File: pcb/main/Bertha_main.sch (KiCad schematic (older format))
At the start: 78 parts, among them J1 RJ12, J12 AudioJack3_SwitchTR, J2 Conn_Coaxial_Power, J3 Conn_02x03_Odd_Even, J4 RJ12, J5 AudioJack3_SwitchTR, J6 SJ, J7 Conn_01x01, J8 Conn_01x01, Q1 ZXMS6004, Q2 ZXMS6004, Q3 MJH6284, Q5 ZXMS6004, Q6 ZXMS6004, Q7 ZXMS6004, U1 DS18B20, U2 ATMEGA32U4-AU, X1 MINI-USB-SCHIELD-32005-201, Y1 Crystal

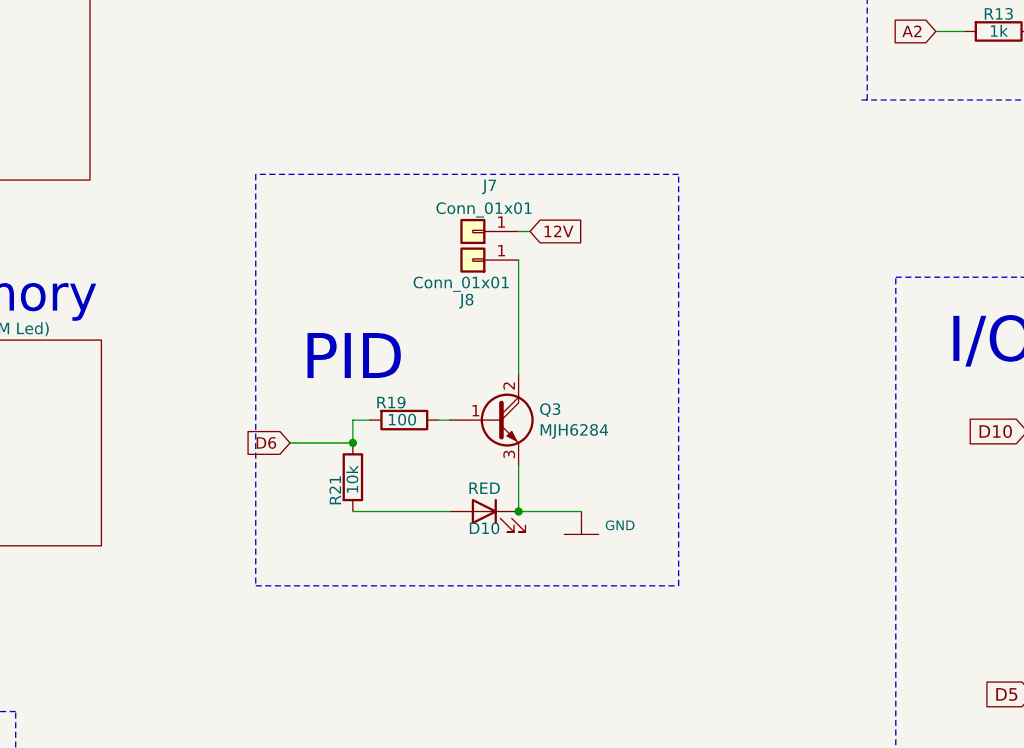
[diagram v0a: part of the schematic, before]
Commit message: Changed MJH6284 darlington transistor for two PB80N03S4L03 MOSFETs
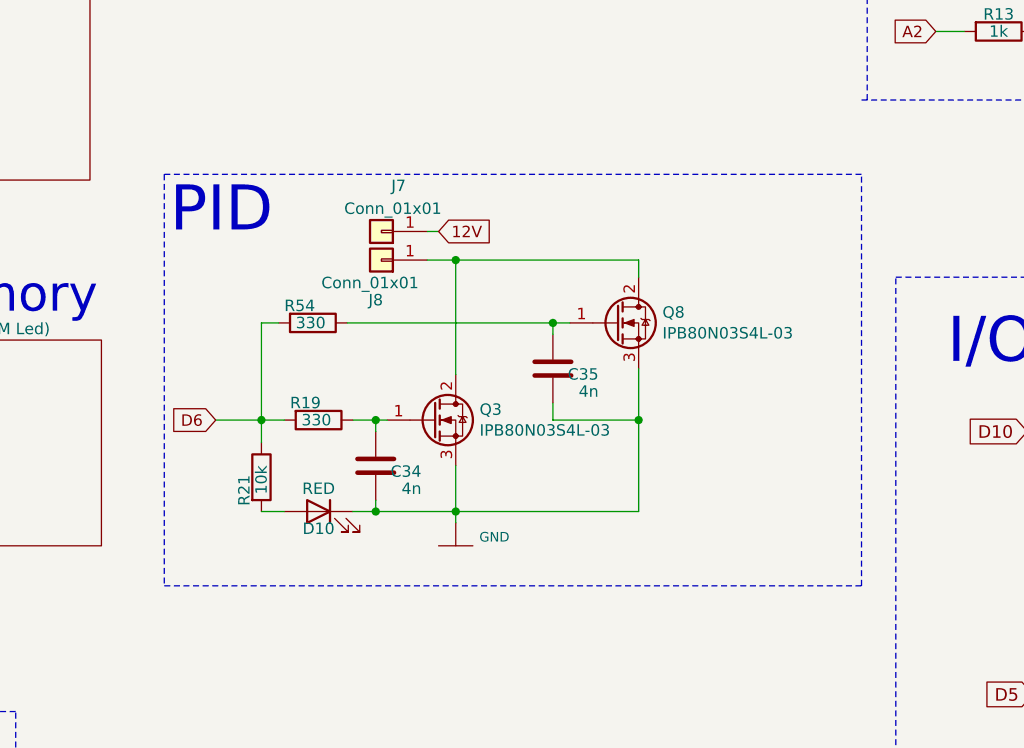
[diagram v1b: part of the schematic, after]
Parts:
- removed Q3: MJH6284, Package_TO_SOT_THT:TO-247-3_Vertical, symbol Device:Q_NPN_Darlington_BCE
- added C34, C35: 4n, Capacitor_SMD:C_0805_2012Metric_Pad1.15x1.40mm_HandSolder, symbol Device:C
- added Q3, Q8: IPB80N03S4L-03, Package_TO_SOT_SMD:TO-263-2, symbol Bertha_main:IPB80N03S4L-03
- added R54: 330, Resistor_SMD:R_0805_2012Metric_Pad1.15x1.40mm_HandSolder, symbol Device:R
- R19: value 100 -> 330
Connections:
- net D6: now also R54.2
- net at J8.1 (Pin_1): now also Q3.2 (D), Q8.2 (D)
- net at R19.1: now also C34.1, Q3.1 (G)
- net at D10.1 (K): now also C34.2, C35.2, Q3.3 (S), Q8.3 (S)
- new net: C35.1, Q8.1 (G), R54.1
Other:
- moved on the sheet: D10, J7, J8, R19, R21
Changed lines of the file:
@@
 	0    1    1    0
 $EndComp
-Text GLabel 9175 6275 2    50   Input ~ 0
+Text GLabel 8775 6275 2    50   Input ~ 0
 12V
 Wire Notes Line
@@
 Wire Notes Line
 	10550 950  10550 2175
-Wire Notes Line
-	7975 7825 9825 7825
-Wire Wire Line
-	8125 7200 8400 7200
-Wire Wire Line
-	9125 6400 9125 6900
-Wire Wire Line
-	9125 7500 9400 7500
-Wire Wire Line
-	9125 7300 9125 7500
+Wire Wire Line
+	8400 7500 8500 7500
 $Comp
 L Device:R R?
 U 1 1 5E02FA68
-P 8400 7350
+P 8000 7350
 AR Path="/5E0D7B15/5E02FA68" Ref="R?"  Part="1"
 AR Path="/5E02FA68" Ref="R21"  Part="1"
-F 0 "R21" V 8325 7225 50  0000 L CNN
-F 1 "10k" V 8400 7275 50  0000 L CNN
-F 2 "Resistor_SMD:R_0805_2012Metric_Pad1.15x1.40mm_HandSolder" V 8330 7350 50  0001 C CNN
-F 3 "~" H 8400 7350 50  0001 C CNN
-	1    8400 7350
-	1    0    0    -1
-$EndComp
-Text GLabel 8125 7200 0    50   Input ~ 0
+F 0 "R21" V 7925 7225 50  0000 L CNN
+F 1 "10k" V 8000 7275 50  0000 L CNN
+F 2 "Resistor_SMD:R_0805_2012Metric_Pad1.15x1.40mm_HandSolder" V 7930 7350 50  0001 C CNN
+F 3 "~" H 8000 7350 50  0001 C CNN
+	1    8000 7350
+	1    0    0    -1
+$EndComp
+Text GLabel 7800 7100 0    50   Input ~ 0
 D6
-Text Notes 8175 6950 0    197  ~ 0
+Text Notes 7600 6300 0    197  ~ 0
 PID
 Wire Notes Line
@@
 L Connector_Generic:Conn_01x01 J8
 U 1 1 5DEEE6F7
-P 8925 6400
-F 0 "J8" H 8950 6575 50  0000 C CNN
-F 1 "Conn_01x01" H 8975 6500 50  0000 C CNN
-F 2 "Connector_Wire:SolderWirePad_1x01_SMD_5x10mm" H 8925 6400 50  0001 C CNN
-F 3 "~" H 8925 6400 50  0001 C CNN
-	1    8925 6400
+P 8525 6400
+F 0 "J8" H 8550 6575 50  0000 C CNN
+F 1 "Conn_01x01" H 8575 6500 50  0000 C CNN
+F 2 "Connector_Wire:SolderWirePad_1x01_SMD_5x10mm" H 8525 6400 50  0001 C CNN
+F 3 "~" H 8525 6400 50  0001 C CNN
+	1    8525 6400
 	-1   0    0    1
 $EndComp
@@
 L Connector_Generic:Conn_01x01 J7
 U 1 1 5DEF8E40
-P 8925 6275
-F 0 "J7" H 8850 6075 50  0000 C CNN
-F 1 "Conn_01x01" H 8875 6175 50  0000 C CNN
-F 2 "Connector_Wire:SolderWirePad_1x01_SMD_5x10mm" H 8925 6275 50  0001 C CNN
-F 3 "~" H 8925 6275 50  0001 C CNN
-	1    8925 6275
+P 8525 6275
+F 0 "J7" H 8450 6075 50  0000 C CNN
+F 1 "Conn_01x01" H 8475 6175 50  0000 C CNN
+F 2 "Connector_Wire:SolderWirePad_1x01_SMD_5x10mm" H 8525 6275 50  0001 C CNN
+F 3 "~" H 8525 6275 50  0001 C CNN
+	1    8525 6275
 	-1   0    0    1
 $EndComp
 Wire Wire Line
-	9125 6275 9175 6275
+	8725 6275 8775 6275
 $Comp
 L Mechanical:MountingHole H3
@@
 L Device:LED D?
 U 1 1 5E92F43F
-P 8975 7500
+P 8250 7500
 AR Path="/5E0005EE/5E92F43F" Ref="D?"  Part="1"
 AR Path="/5E92F43F" Ref="D10"  Part="1"
-F 0 "D10" H 8975 7425 50  0000 C CNN
-F 1 "RED" H 8975 7600 50  0000 C CNN
-F 2 "LED_SMD:LED_0805_2012Metric_Pad1.15x1.40mm_HandSolder" H 8975 7500 50  0001 C CNN
-F 3 "~" H 8975 7500 50  0001 C CNN
-	1    8975 7500
+F 0 "D10" H 8250 7425 50  0000 C CNN
+F 1 "RED" H 8250 7600 50  0000 C CNN
+F 2 "LED_SMD:LED_0805_2012Metric_Pad1.15x1.40mm_HandSolder" H 8250 7500 50  0001 C CNN
+F 3 "~" H 8250 7500 50  0001 C CNN
+	1    8250 7500
 	-1   0    0    -1
 $EndComp
-Connection ~ 9125 7500
 $Comp
 L Connector:Conn_Coaxial_Power J2
@@
 	7950 3200 7950 5150
 Wire Notes Line
-	7975 6025 7975 7825
-Wire Notes Line
-	9825 7825 9825 6025
-Wire Notes Line
-	9825 6025 7975 6025
+	7575 6025 7575 7825
+Wire Notes Line
+	10625 7825 10625 6025
 Wire Notes Line
 	5250 3275 5250 7550
@@
 	5600 6975 5850 6975
 $Comp
-L Bertha_main-eagle-import:GND #020
-U 1 1 5E54DBF3
-P 9400 7600
-F 0 "#020" H 9450 7650 50  0001 C CNN
-F 1 "GND" H 9503 7638 42  0000 L CNN
-F 2 "" H 9400 7600 50  0001 C CNN
-F 3 "" H 9400 7600 50  0001 C CNN
-	1    9400 7600
-	1    0    0    -1
-$EndComp
-$Comp
 L Bertha_main-eagle-import:GND #U05
 U 1 1 5E54E01E
@@
 Wire Wire Line
 	11675 8300 11875 8300
-$Comp
-L Device:Q_NPN_Darlington_BCE Q3
-U 1 1 5E1B6F78
-P 9025 7100
-F 0 "Q3" H 9215 7146 50  0000 L CNN
-F 1 "MJH6284" H 9215 7055 50  0000 L CNN
-F 2 "Package_TO_SOT_THT:TO-247-3_Vertical" H 9225 7200 50  0001 C CNN
-F 3 "~" H 9025 7100 50  0001 C CNN
-	1    9025 7100
-	1    0    0    -1
-$EndComp
-Wire Wire Line
-	8400 7200 8400 7100
-Connection ~ 8400 7200
-Wire Wire Line
-	8400 7500 8825 7500
+Wire Wire Line
+	8000 7200 8000 7100
+Wire Wire Line
+	8000 7500 8100 7500
 $Comp
 L Device:R R?
 U 1 1 5E2163A8
-P 8625 7100
+P 8250 7100
 AR Path="/5E0D7B15/5E2163A8" Ref="R?"  Part="1"
 AR Path="/5E2163A8" Ref="R19"  Part="1"
-F 0 "R19" V 8550 6975 50  0000 L CNN
-F 1 "100" V 8625 7025 50  0000 L CNN
-F 2 "Resistor_SMD:R_0805_2012Metric_Pad1.15x1.40mm_HandSolder" V 8555 7100 50  0001 C CNN
-F 3 "~" H 8625 7100 50  0001 C CNN
-	1    8625 7100
-	0    1    1    0
-$EndComp
-Wire Wire Line
-	8475 7100 8400 7100
-Wire Wire Line
-	8775 7100 8825 7100
+F 0 "R19" V 8175 6975 50  0000 L CNN
+F 1 "330" V 8250 7025 50  0000 L CNN
+F 2 "Resistor_SMD:R_0805_2012Metric_Pad1.15x1.40mm_HandSolder" V 8180 7100 50  0001 C CNN
+F 3 "~" H 8250 7100 50  0001 C CNN
+	1    8250 7100
+	0    1    1    0
+$EndComp
+Wire Wire Line
+	8100 7100 8000 7100
 Text Label 4275 6450 0    50   ~ 0
 D12
@@
 Wire Wire Line
 	12025 4050 12550 4050
+$Comp
+L Bertha_main:IPB80N03S4L-03 Q8
+U 1 1 5F48D945
+P 9550 6675
+F 0 "Q8" H 9754 6721 50  0000 L CNN
+F 1 "IPB80N03S4L-03" H 9754 6630 50  0000 L CNN
+F 2 "Package_TO_SOT_SMD:TO-263-2" H 9750 6600 50  0001 L CIN
+F 3 "https://www.infineon.com/dgdl/Infineon-IPB80N03S4L-03-DataSheet-v02_01-EN.pdf?fileId=5546d4626cb27db2016ccd4c03921b4c" H 9550 6675 50  0001 L CNN
+	1    9550 6675
+	1    0    0    -1
+$EndComp
+$Comp
+L Device:C C?
+U 1 1 5F4777DE
+P 9275 6875
+AR Path="/5E02557B/5F4777DE" Ref="C?"  Part="1"
+AR Path="/5F4777DE" Ref="C35"  Part="1"
+F 0 "C35" H 9075 6850 50  0000 L CNN
+F 1 "4n" H 9075 6775 50  0000 L CNN
+F 2 "Capacitor_SMD:C_0805_2012Metric_Pad1.15x1.40mm_HandSolder" H 9313 6725 50  0001 C CNN
+F 3 "~" H 9275 6875 50  0001 C CNN
+	1    9275 6875
+	-1   0    0    -1
+$EndComp
+$Comp
+L Device:R R?
+U 1 1 5F4B2886
+P 8225 6675
+AR Path="/5E0D7B15/5F4B2886" Ref="R?"  Part="1"
+AR Path="/5F4B2886" Ref="R54"  Part="1"
+F 0 "R54" V 8150 6550 50  0000 L CNN
+F 1 "330" V 8225 6600 50  0000 L CNN
+F 2 "Resistor_SMD:R_0805_2012Metric_Pad1.15x1.40mm_HandSolder" V 8155 6675 50  0001 C CNN
+F 3 "~" H 8225 6675 50  0001 C CNN
+	1    8225 6675
+	0    1    1    0
+$EndComp
+Wire Wire Line
+	9350 6675 9275 6675
+Wire Wire Line
+	9275 6725 9275 6675
+Connection ~ 9275 6675
+Wire Wire Line
+	9275 6675 8375 6675
+Wire Wire Line
+	9275 7025 9275 7100
+Wire Wire Line
+	9275 7100 9650 7100
+Wire Wire Line
+	9650 7100 9650 6875
+Wire Wire Line
+	8075 6675 8000 6675
+Wire Wire Line
+	8000 6675 8000 7100
+Connection ~ 8000 7100
+$Comp
+L Device:C C?
+U 1 1 5F59928D
+P 8500 7300
+AR Path="/5E02557B/5F59928D" Ref="C?"  Part="1"
+AR Path="/5F59928D" Ref="C34"  Part="1"
+F 0 "C34" H 8300 7275 50  0000 L CNN
+F 1 "4n" H 8300 7200 50  0000 L CNN
+F 2 "Capacitor_SMD:C_0805_2012Metric_Pad1.15x1.40mm_HandSolder" H 8538 7150 50  0001 C CNN
+F 3 "~" H 8500 7300 50  0001 C CNN
+	1    8500 7300
+	-1   0    0    -1
+$EndComp
+Wire Wire Line
+	8400 7100 8500 7100
+Wire Wire Line
+	8500 7150 8500 7100
+Connection ~ 8500 7100
+Wire Wire Line
+	8500 7100 8550 7100
+$Comp
+L Bertha_main:IPB80N03S4L-03 Q3
+U 1 1 5F62A5B7
+P 8750 7100
+F 0 "Q3" H 8954 7146 50  0000 L CNN
+F 1 "IPB80N03S4L-03" H 8954 7055 50  0000 L CNN
+F 2 "Package_TO_SOT_SMD:TO-263-2" H 8950 7025 50  0001 L CIN
+F 3 "https://www.infineon.com/dgdl/Infineon-IPB80N03S4L-03-DataSheet-v02_01-EN.pdf?fileId=5546d4626cb27db2016ccd4c03921b4c" H 8750 7100 50  0001 L CNN
+	1    8750 7100
+	1    0    0    -1
+$EndComp
+Wire Wire Line
+	8500 7450 8500 7500
+Connection ~ 8500 7500
+Wire Wire Line
+	8500 7500 8850 7500
+Wire Wire Line
+	8850 7300 8850 7500
+Wire Wire Line
+	9650 7100 9650 7500
+Connection ~ 9650 7100
+$Comp
+L Bertha_main-eagle-import:GND #020
+U 1 1 5E54DBF3
+P 8850 7650
+F 0 "#020" H 8900 7700 50  0001 C CNN
+F 1 "GND" H 8953 7688 42  0000 L CNN
+F 2 "" H 8850 7650 50  0001 C CNN
+F 3 "" H 8850 7650 50  0001 C CNN
+	1    8850 7650
+	1    0    0    -1
+$EndComp
+Wire Wire Line
+	8850 7550 8850 7500
+Connection ~ 8850 7500
+Wire Wire Line
+	9650 7500 8850 7500
+Wire Wire Line
+	8850 6900 8850 6400
+Wire Wire Line
+	8850 6400 8725 6400
+Wire Wire Line
+	9650 6475 9650 6400
+Wire Wire Line
+	9650 6400 8850 6400
+Connection ~ 8850 6400
+Wire Wire Line
+	7800 7100 8000 7100
+Wire Notes Line
+	7575 7825 10625 7825
+Wire Notes Line
+	7575 6025 10625 6025
 $EndSCHEMATC
